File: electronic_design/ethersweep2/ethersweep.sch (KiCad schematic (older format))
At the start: 68 parts, among them J1 AVR-ISP-6, J2 Conn_01x02_Male, J3 Conn_01x04_Female, J4 Conn_01x02_Male, J5 Conn_01x02_Male, J6 HR911105A, J7 Conn_01x04_Female, J8 AVR-ISP-6, J9 Conn_01x04_Female, M1 Stepper_Motor_bipolar, SW1 SW_Push, U1 ENC28J60x-SS, U2 ATmega328-AU, U3 DRV8825PWPR, U4 AMS1117-3.3, U5 AS5600, Y1 Crystal_25MHz, Y2 Crystal_8MHz

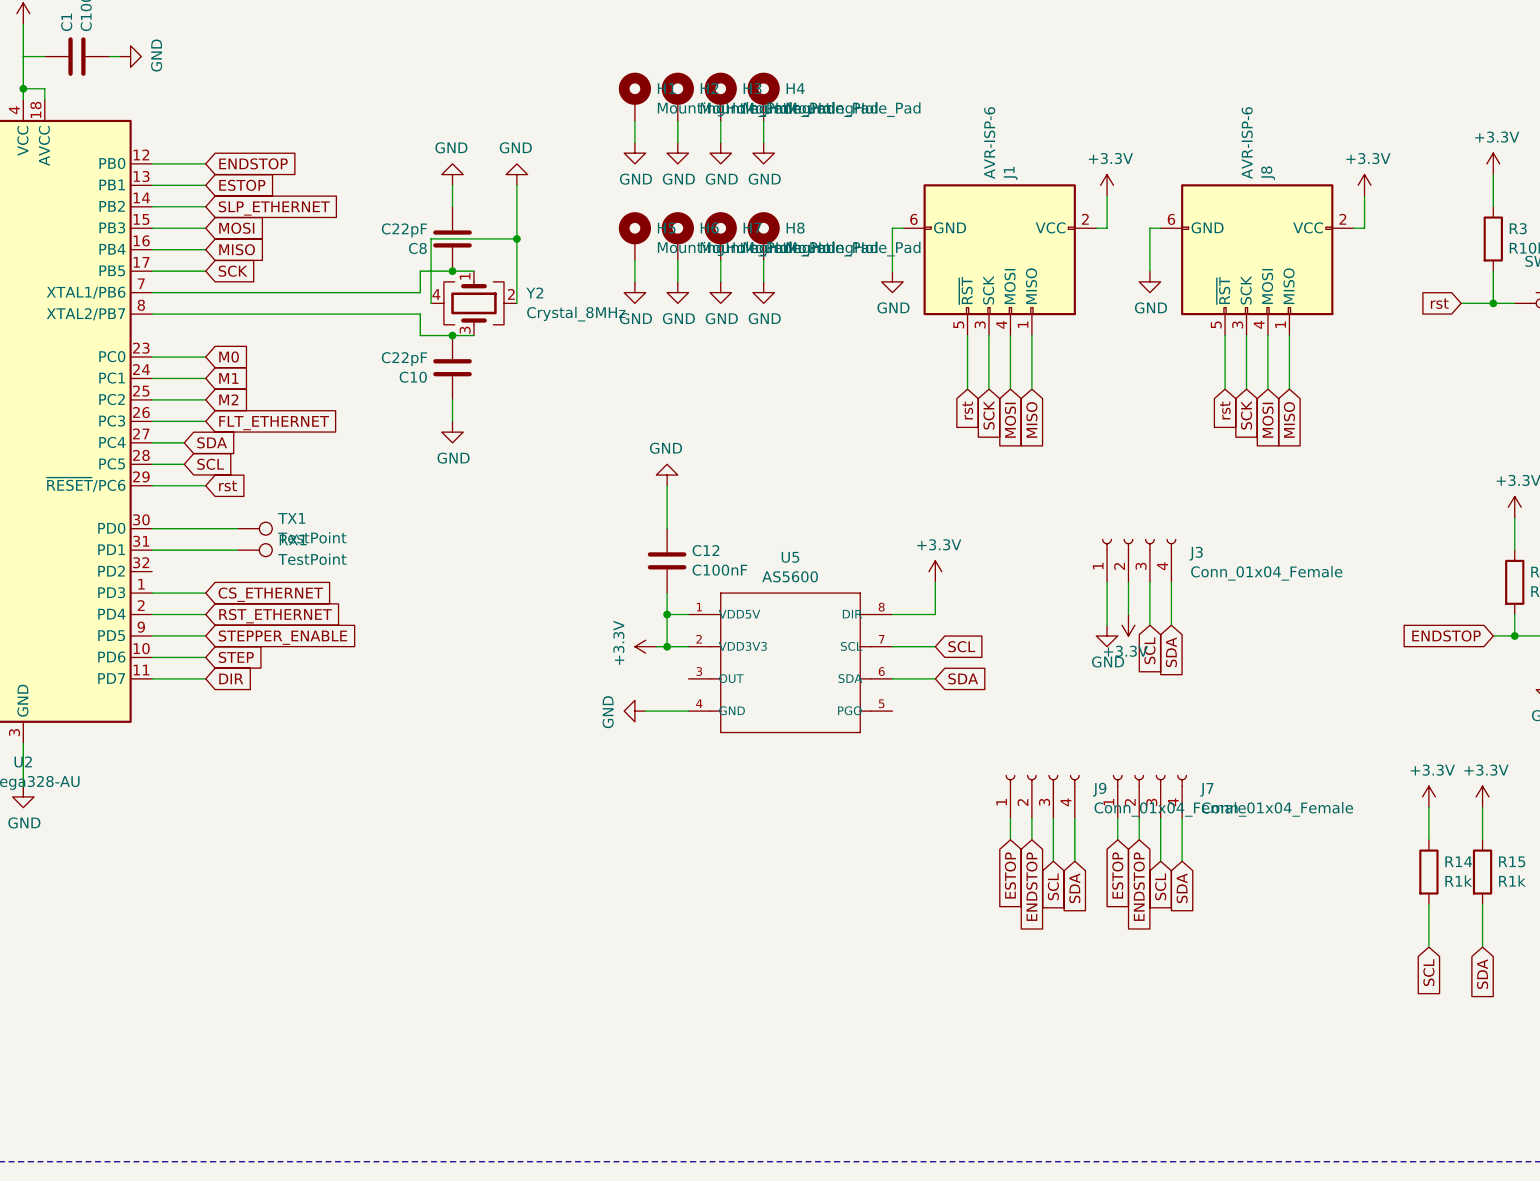
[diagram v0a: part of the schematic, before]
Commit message: design improvements and error fixes
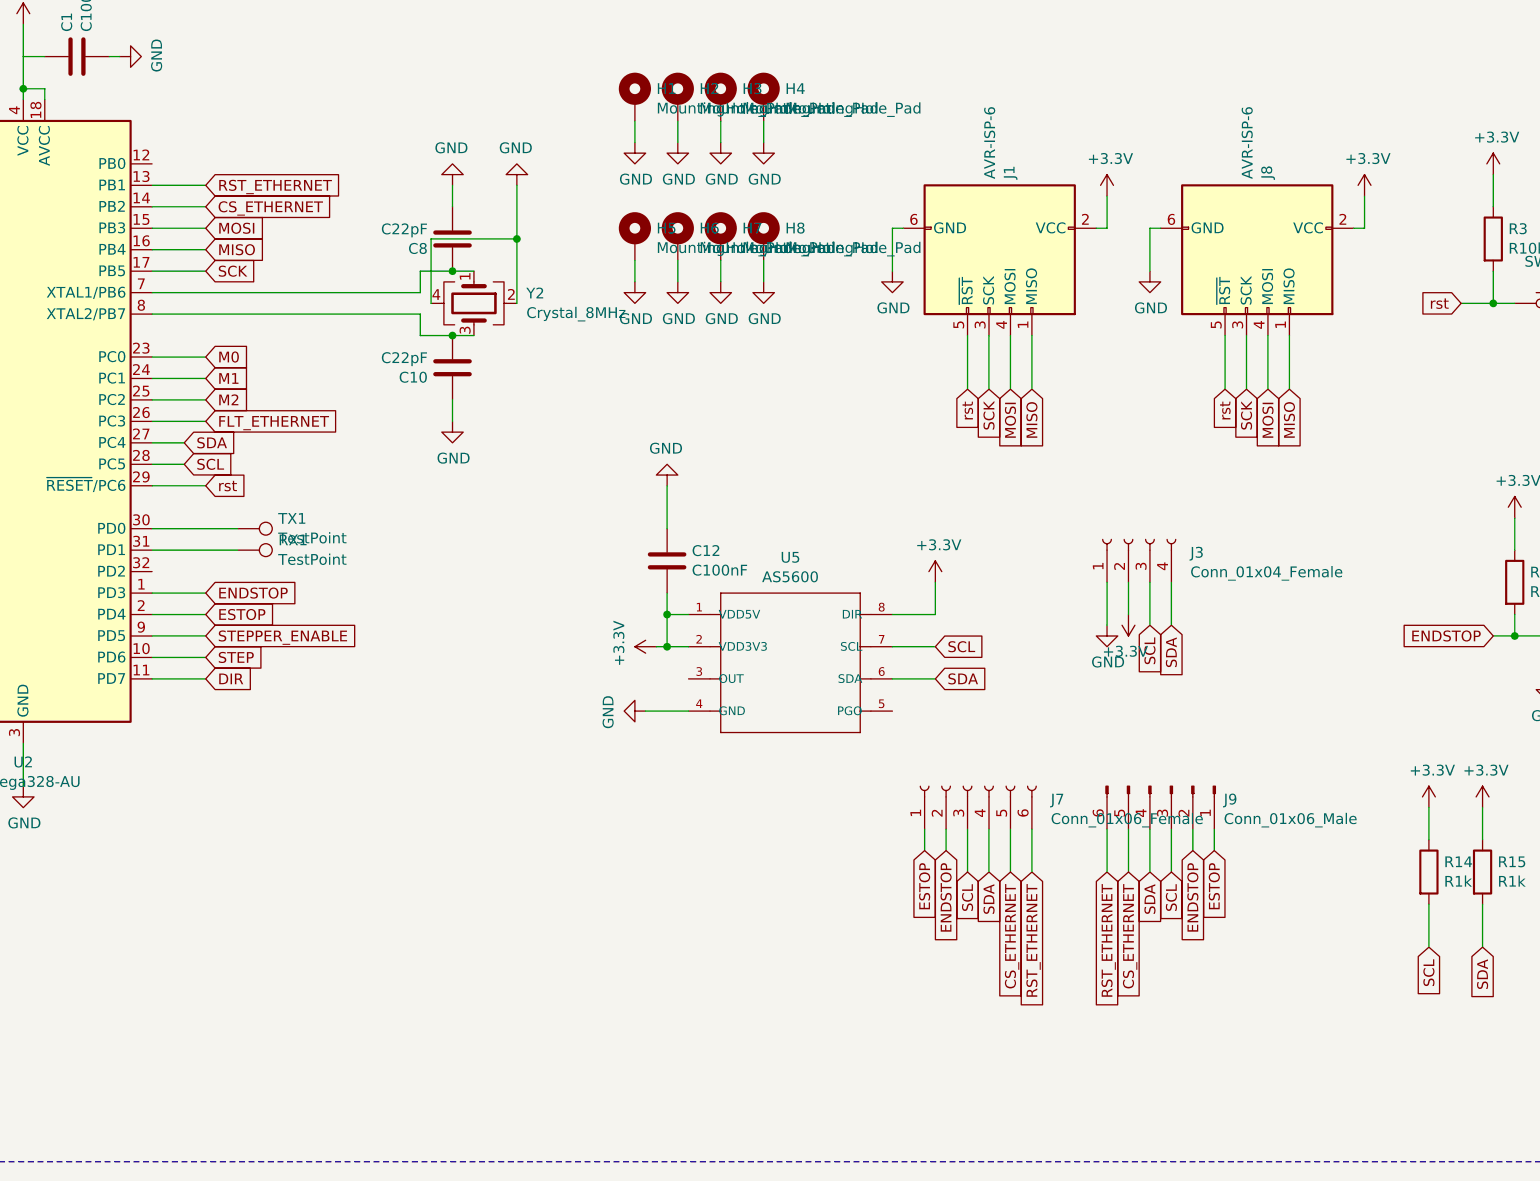
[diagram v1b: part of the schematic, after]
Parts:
- removed J7, J9: Conn_01x04_Female, Connector_PinHeader_2.54mm:PinHeader_1x04_P2.54mm_Vertical, symbol Connector:Conn_01x04_Female
- added J7: Conn_01x06_Female, Connector_PinHeader_2.54mm:PinHeader_1x06_P2.54mm_Vertical, symbol Connector:Conn_01x06_Female
- added J9: Conn_01x06_Male, Connector_PinHeader_2.54mm:PinHeader_1x06_P2.54mm_Vertical, symbol Connector:Conn_01x06_Male
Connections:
- net SLP_ETHERNET is gone; now on net CS_ETHERNET: U2.14 (PB2)
- net CS_ETHERNET: now also J7.5 (Pin_5), J9.5 (Pin_5); no longer U2.1 (PD3)
- net ENDSTOP: now also U2.1 (PD3), J7.2 (Pin_2), J9.2 (Pin_2); no longer U2.12 (PB0)
- net ESTOP: now also U2.2 (PD4), J7.1 (Pin_1), J9.1 (Pin_1); no longer U2.13 (PB1)
- net RST_ETHERNET: now also U2.13 (PB1), J7.6 (Pin_6), J9.6 (Pin_6); no longer U2.2 (PD4)
- net SCL: now also J7.3 (Pin_3), J9.3 (Pin_3)
- net SDA: now also J7.4 (Pin_4), J9.4 (Pin_4)
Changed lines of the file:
@@
 Wire Wire Line
 	8800 1900 8800 2000
-Text GLabel 2200 1250 2    50   Input ~ 0
+Text GLabel 2200 3250 2    50   Input ~ 0
 ENDSTOP
-Text GLabel 2200 1350 2    50   Input ~ 0
+Text GLabel 2200 3350 2    50   Input ~ 0
 ESTOP
 $Comp
@@
 	1950 1650 2200 1650
 Wire Wire Line
-	1950 1250 2200 1250
-Wire Wire Line
-	2200 1350 1950 1350
+	1950 1350 2200 1350
+Wire Wire Line
+	2200 1450 1950 1450
 $Comp
 L AS5600:AS5600 U5
@@
 Wire Wire Line
 	1350 750  1350 900
-Text GLabel 2200 3250 2    50   Input ~ 0
+Text GLabel 2200 1450 2    50   Input ~ 0
 CS_ETHERNET
 Wire Wire Line
 	1950 3250 2200 3250
-Text GLabel 2200 3350 2    50   Input ~ 0
+Text GLabel 2200 1350 2    50   Input ~ 0
 RST_ETHERNET
 Wire Wire Line
@@
 Wire Wire Line
 	1950 2450 2200 2450
-Text GLabel 2200 1450 2    50   Input ~ 0
-SLP_ETHERNET
-Wire Wire Line
-	1950 1450 2200 1450
 $Comp
 L MCU_Microchip_ATmega:ATmega328-AU U2
@@
 $EndComp
 $Comp
-L Connector:Conn_01x04_Female J7
-U 1 1 618AEEEB
-P 6550 4100
-F 0 "J7" V 6488 3812 50  0000 R CNN
-F 1 "Conn_01x04_Female" V 6397 3812 50  0000 R CNN
-F 2 "Connector_PinHeader_2.54mm:PinHeader_1x04_P2.54mm_Vertical" H 6550 4100 50  0001 C CNN
-F 3 "~" H 6550 4100 50  0001 C CNN
-	1    6550 4100
-	0    -1   -1   0
-$EndComp
-Text GLabel 6750 4500 3    50   Input ~ 0
-SDA
-Text GLabel 6650 4500 3    50   Input ~ 0
-SCL
-Wire Wire Line
-	6650 4300 6650 4500
-Wire Wire Line
-	6750 4500 6750 4300
-Wire Wire Line
-	6550 4400 6550 4300
-Text GLabel 6550 4400 3    50   Input ~ 0
-ENDSTOP
-Wire Wire Line
-	6450 4400 6450 4300
-Text GLabel 6450 4400 3    50   Input ~ 0
-ESTOP
-$Comp
 L Mechanical:MountingHole_Pad H8
 U 1 1 6192C950
@@
 Wire Wire Line
 	4200 1700 4200 1800
-$Comp
-L Connector:Conn_01x04_Female J9
-U 1 1 61992053
-P 6050 4100
-F 0 "J9" V 5988 3812 50  0000 R CNN
-F 1 "Conn_01x04_Female" V 5897 3812 50  0000 R CNN
-F 2 "Connector_PinHeader_2.54mm:PinHeader_1x04_P2.54mm_Vertical" H 6050 4100 50  0001 C CNN
-F 3 "~" H 6050 4100 50  0001 C CNN
-	1    6050 4100
-	0    -1   -1   0
-$EndComp
-Text GLabel 6250 4500 3    50   Input ~ 0
+Text GLabel 5850 4550 3    50   Input ~ 0
 SDA
-Text GLabel 6150 4500 3    50   Input ~ 0
+Text GLabel 5750 4550 3    50   Input ~ 0
 SCL
 Wire Wire Line
-	6150 4300 6150 4500
-Wire Wire Line
-	6250 4500 6250 4300
-Wire Wire Line
-	6050 4400 6050 4300
-Text GLabel 6050 4400 3    50   Input ~ 0
+	5750 4350 5750 4550
+Wire Wire Line
+	5850 4550 5850 4350
+Wire Wire Line
+	5650 4450 5650 4350
+Text GLabel 5650 4450 3    50   Input ~ 0
 ENDSTOP
 Wire Wire Line
-	5950 4400 5950 4300
-Text GLabel 5950 4400 3    50   Input ~ 0
+	5550 4450 5550 4350
+Text GLabel 5550 4450 3    50   Input ~ 0
 ESTOP
 Wire Wire Line
@@
 Wire Notes Line
 	11450 8650 11450 4750
+Text GLabel 6050 4550 3    50   Input ~ 0
+RST_ETHERNET
+Text GLabel 5950 4550 3    50   Input ~ 0
+CS_ETHERNET
+$Comp
+L Connector:Conn_01x06_Female J7
+U 1 1 61DB5EEA
+P 5750 4150
+F 0 "J7" V 5688 3762 50  0000 R CNN
+F 1 "Conn_01x06_Female" V 5597 3762 50  0000 R CNN
+F 2 "Connector_PinHeader_2.54mm:PinHeader_1x06_P2.54mm_Vertical" H 5750 4150 50  0001 C CNN
+F 3 "~" H 5750 4150 50  0001 C CNN
+	1    5750 4150
+	0    -1   -1   0
+$EndComp
+$Comp
+L Connector:Conn_01x06_Male J9
+U 1 1 61DB8F12
+P 6700 4150
+F 0 "J9" V 6762 4394 50  0000 L CNN
+F 1 "Conn_01x06_Male" V 6853 4394 50  0000 L CNN
+F 2 "Connector_PinHeader_2.54mm:PinHeader_1x06_P2.54mm_Vertical" H 6700 4150 50  0001 C CNN
+F 3 "~" H 6700 4150 50  0001 C CNN
+	1    6700 4150
+	0    1    1    0
+$EndComp
+Wire Wire Line
+	5950 4550 5950 4350
+Wire Wire Line
+	6050 4550 6050 4350
+Text GLabel 6600 4550 3    50   Input ~ 0
+SDA
+Text GLabel 6700 4550 3    50   Input ~ 0
+SCL
+Wire Wire Line
+	6700 4350 6700 4550
+Wire Wire Line
+	6600 4550 6600 4350
+Wire Wire Line
+	6800 4450 6800 4350
+Text GLabel 6800 4450 3    50   Input ~ 0
+ENDSTOP
+Wire Wire Line
+	6900 4450 6900 4350
+Text GLabel 6900 4450 3    50   Input ~ 0
+ESTOP
+Text GLabel 6400 4550 3    50   Input ~ 0
+RST_ETHERNET
+Text GLabel 6500 4550 3    50   Input ~ 0
+CS_ETHERNET
+Wire Wire Line
+	6500 4550 6500 4350
+Wire Wire Line
+	6400 4550 6400 4350
 $EndSCHEMATC
